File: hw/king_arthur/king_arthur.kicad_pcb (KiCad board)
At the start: 2 copper layers, 70 x 50 mm, 0 parts

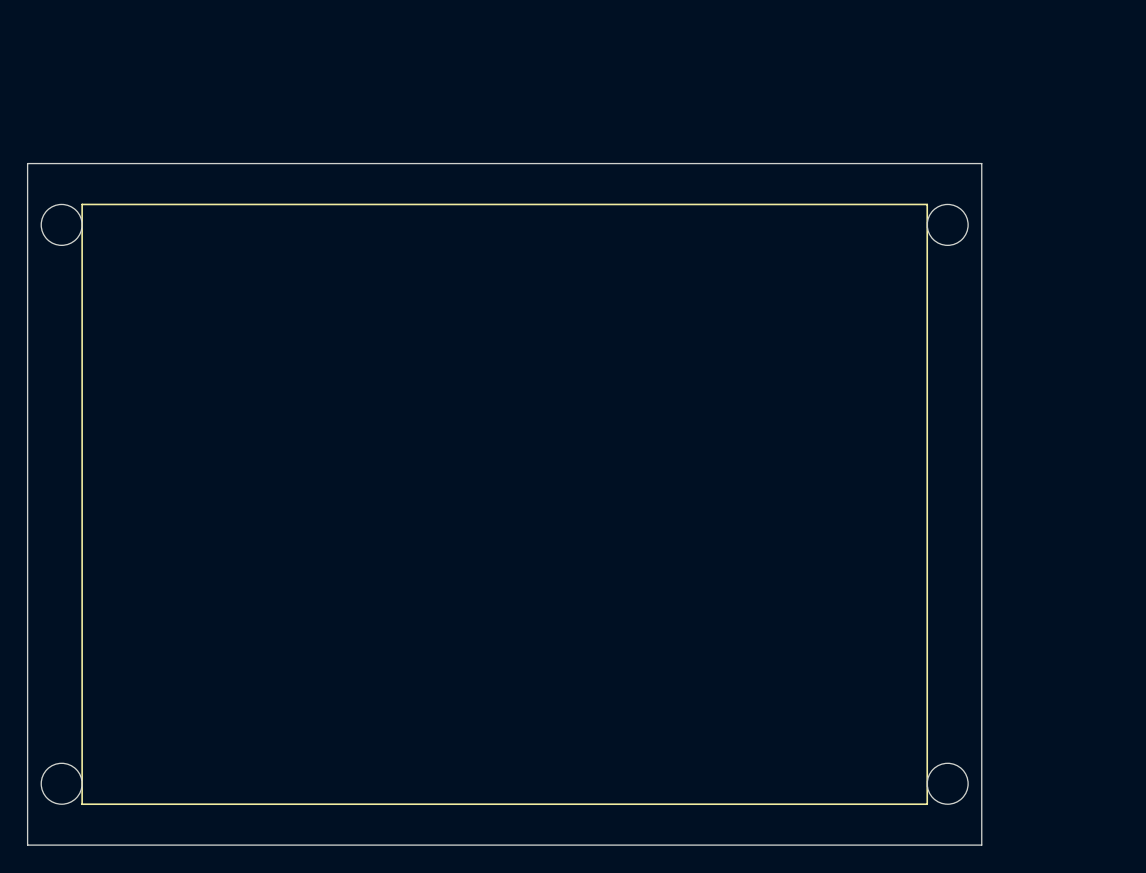
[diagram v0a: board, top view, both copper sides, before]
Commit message: shematic and pcb done
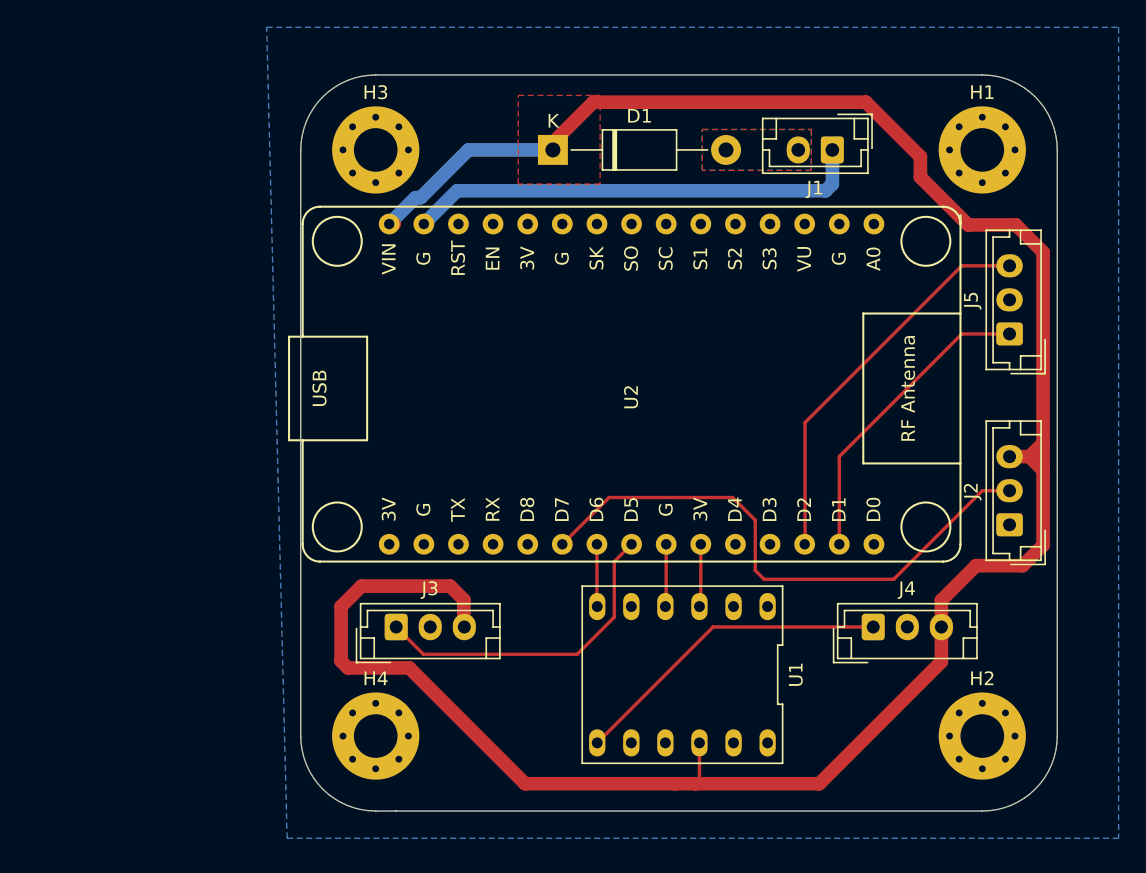
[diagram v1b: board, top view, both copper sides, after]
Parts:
- added D1: D, Diode_THT:D_DO-41_SOD81_P12.70mm_Horizontal, F.Cu at (88.5, 39.0)
- added H1: MountingHole_Pad, MountingHole:MountingHole_3.2mm_M3_Pad_Via, F.Cu at (120.0, 39.0)
- added H2: MountingHole_Pad, MountingHole:MountingHole_3.2mm_M3_Pad_Via, F.Cu at (120.0, 82.0)
- added H3: MountingHole_Pad, MountingHole:MountingHole_3.2mm_M3_Pad_Via, F.Cu at (75.5, 39.0)
- added H4: MountingHole_Pad, MountingHole:MountingHole_3.2mm_M3_Pad_Via, F.Cu at (75.5, 82.0)
- added J1: POWER, Connector_JST:JST_EH_B2B-EH-A_1x02_P2.50mm_Vertical, F.Cu at (109.0, 39.0)
- added J2: PIR sensor, Connector_JST:JST_EH_B3B-EH-A_1x03_P2.50mm_Vertical, F.Cu at (122.0, 66.5)
- added J3: IR sensor, Connector_JST:JST_EH_B3B-EH-A_1x03_P2.50mm_Vertical, F.Cu at (77.0, 74.0)
- added J4: Servo motor, Connector_JST:JST_EH_B3B-EH-A_1x03_P2.50mm_Vertical, F.Cu at (112.0, 74.0)
- added J5: Descrete sensor of SWORD block pin state, Connector_JST:JST_EH_B3B-EH-A_1x03_P2.50mm_Vertical, F.Cu at (122.0, 52.5)
- added U1: Logisshifter, king_arthur:DIP-12_393_ELL, F.Cu at (98.0, 77.5)
- added U2: NodeMCU_1.0_(ESP-12E), ESP8266:ESP12F-Devkit-V3, F.Cu at (93.0, 56.5)
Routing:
- net +5V: track 0.00 -> 167.9 mm
- net PIR: track 0.00 -> 41.6 mm
- net GND: track 0.00 -> 33.7 mm
- net PIN_IN: track 0.00 -> 28.7 mm
- net IR: track 0.00 -> 23.8 mm
- net Motor: track 0.00 -> 23.8 mm
- net PIN_OUT: track 0.00 -> 22.7 mm
- net Net-(U1-Pad3): track 0.00 -> 4.61 mm
- net Net-(U1-Pad4): track 0.00 -> 4.59 mm
- net Net-(U1-Pad6): track 0.00 -> 4.58 mm
- added copper zone on F.Cu, net +5V
- added copper zone on B.Cu, net GND
- added copper zone on B.Cu, net Net-(D1-Pad2)
- added copper zone on F.Cu, net Net-(D1-Pad2)
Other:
- board size 70 x 50 mm -> 55.5 x 54 mm
